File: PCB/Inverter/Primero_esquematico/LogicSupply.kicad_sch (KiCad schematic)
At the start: 32 parts, among them U23 LM25180QNGURQ1, U24 LP5907QMFX-3.3Q1, U25 TLV76733QWDRBRQ1, U26 TPS7A2050PDBVR, U27 REF2030-Q1

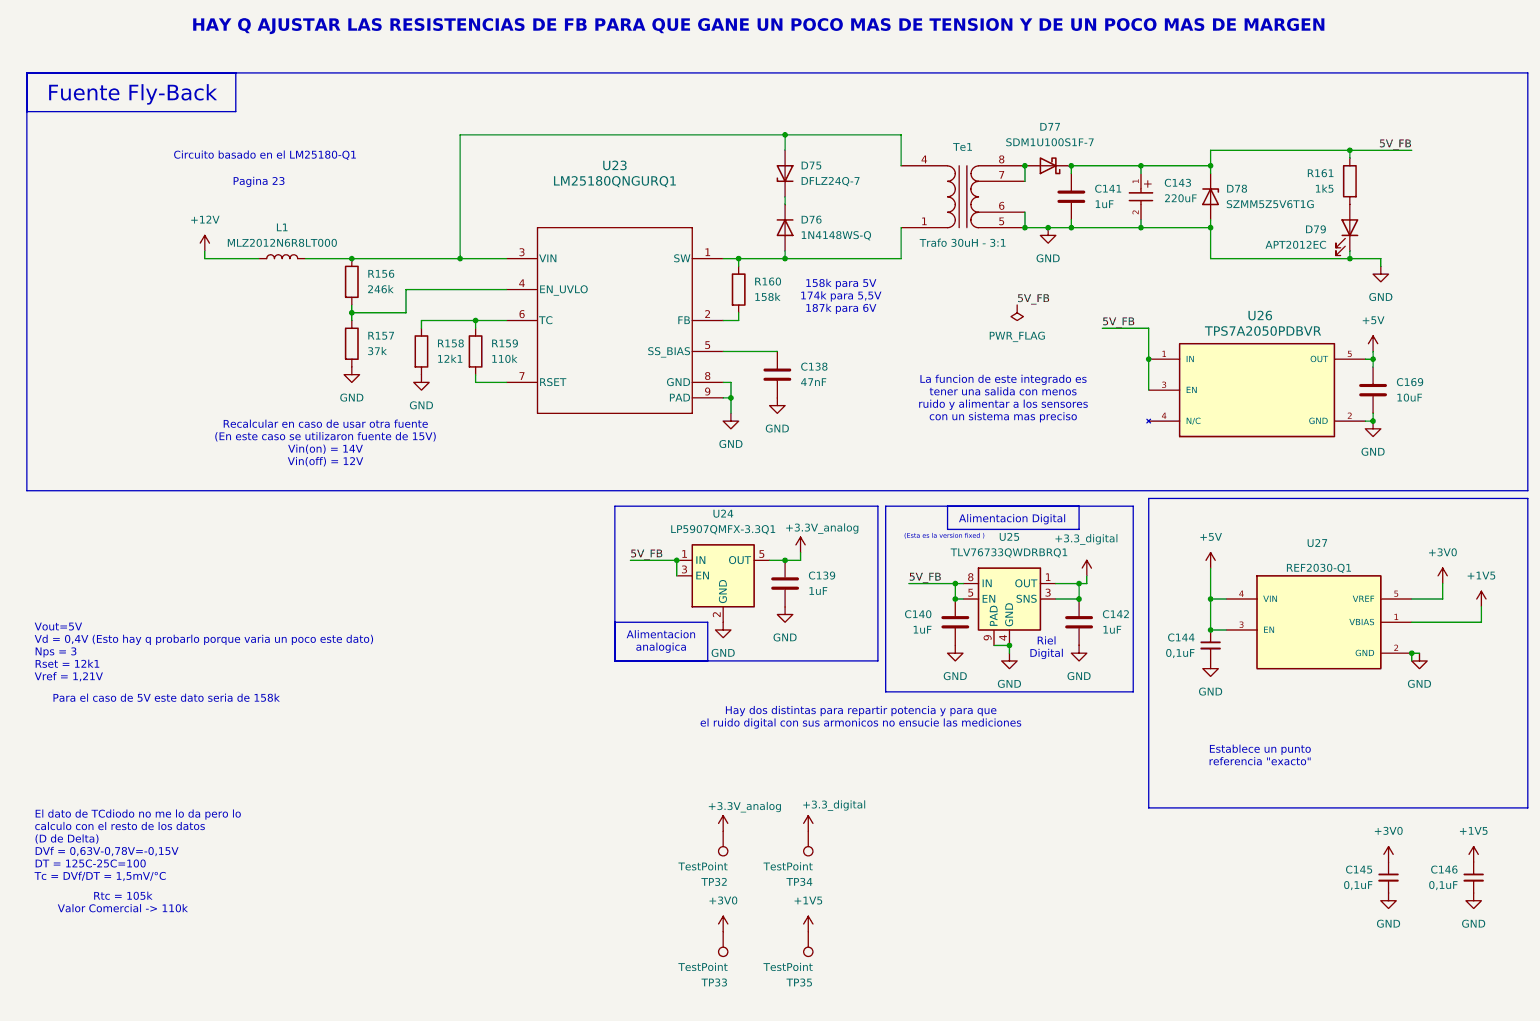
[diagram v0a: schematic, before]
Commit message: a
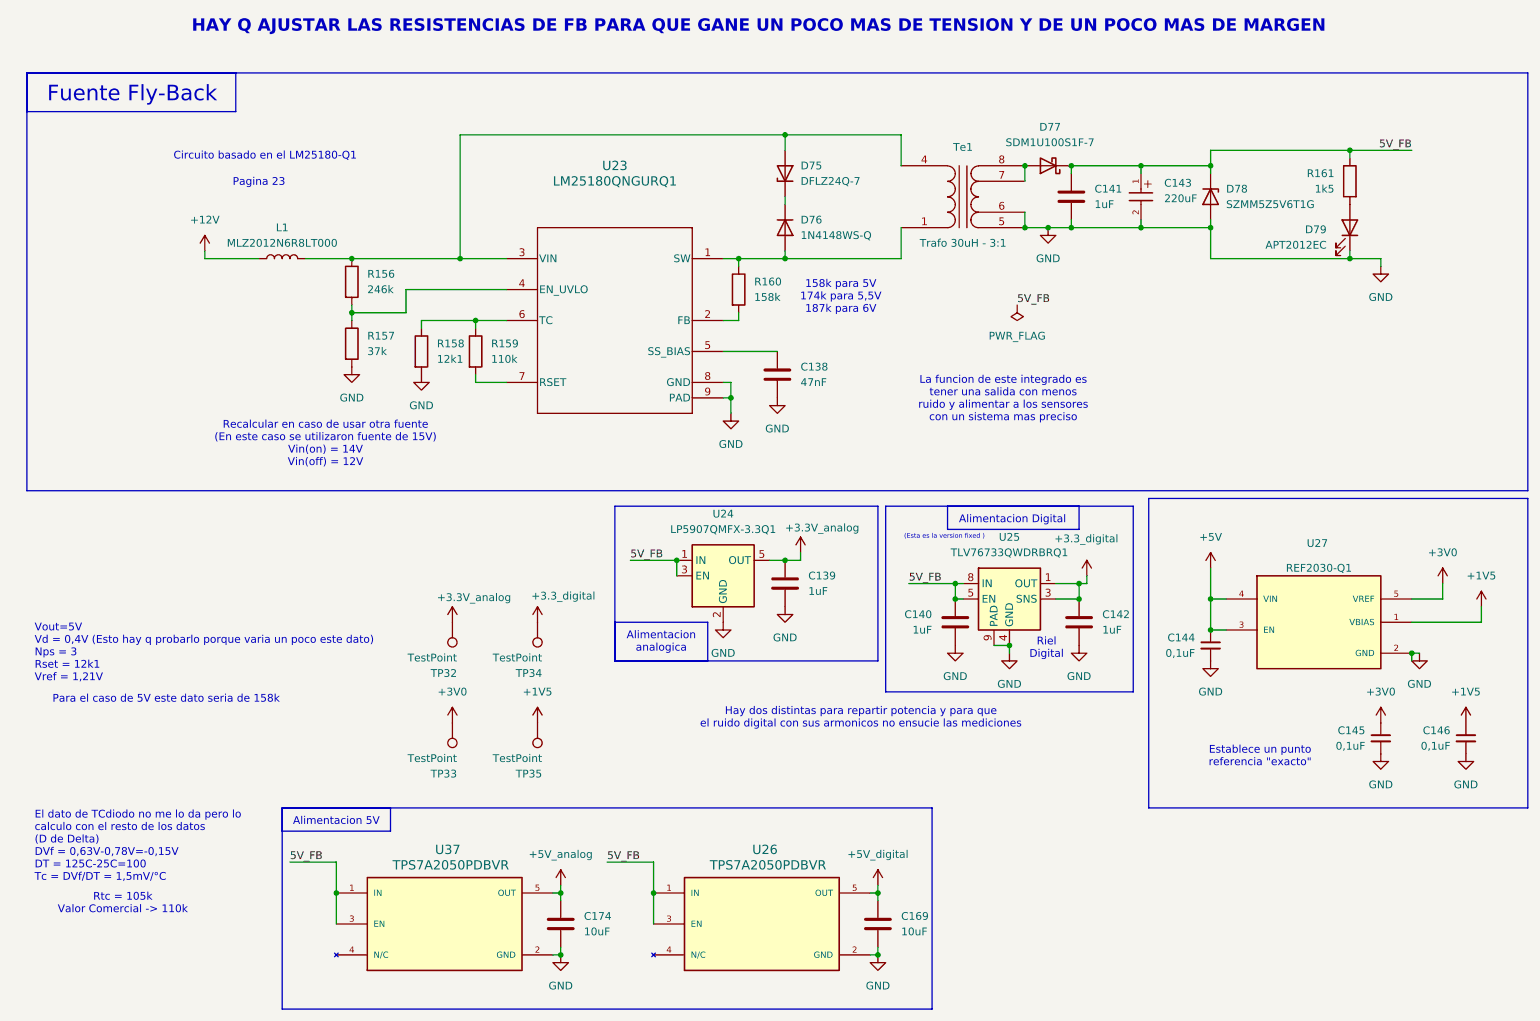
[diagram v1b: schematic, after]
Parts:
- added C174: 10uF, Capacitor_SMD:C_0805_2012Metric, symbol Device:C
- added U37: TPS7A2050PDBVR, Snapeda:DBV0005A-IPC_A, symbol Snapeda:TPS7A2050PDBVR
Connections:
- net +5V: no longer C169.2, U26.5 (OUT)
- net 5V_FB: now also U37.1 (IN), U37.3 (EN)
- net GND: now also C174.1, U37.2 (GND)
- new net +5V_analog: C174.2, U37.5 (OUT)
- new net +5V_digital: C169.2, U26.5 (OUT)
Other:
- note added: "Alimentacion 5V"
- moved on the sheet: C145, C146, TP32, TP33, TP34, TP35
